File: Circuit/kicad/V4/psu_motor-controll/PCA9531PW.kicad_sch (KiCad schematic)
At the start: 15 parts, among them J1 Conn_01x12, U3 PCA9685PW

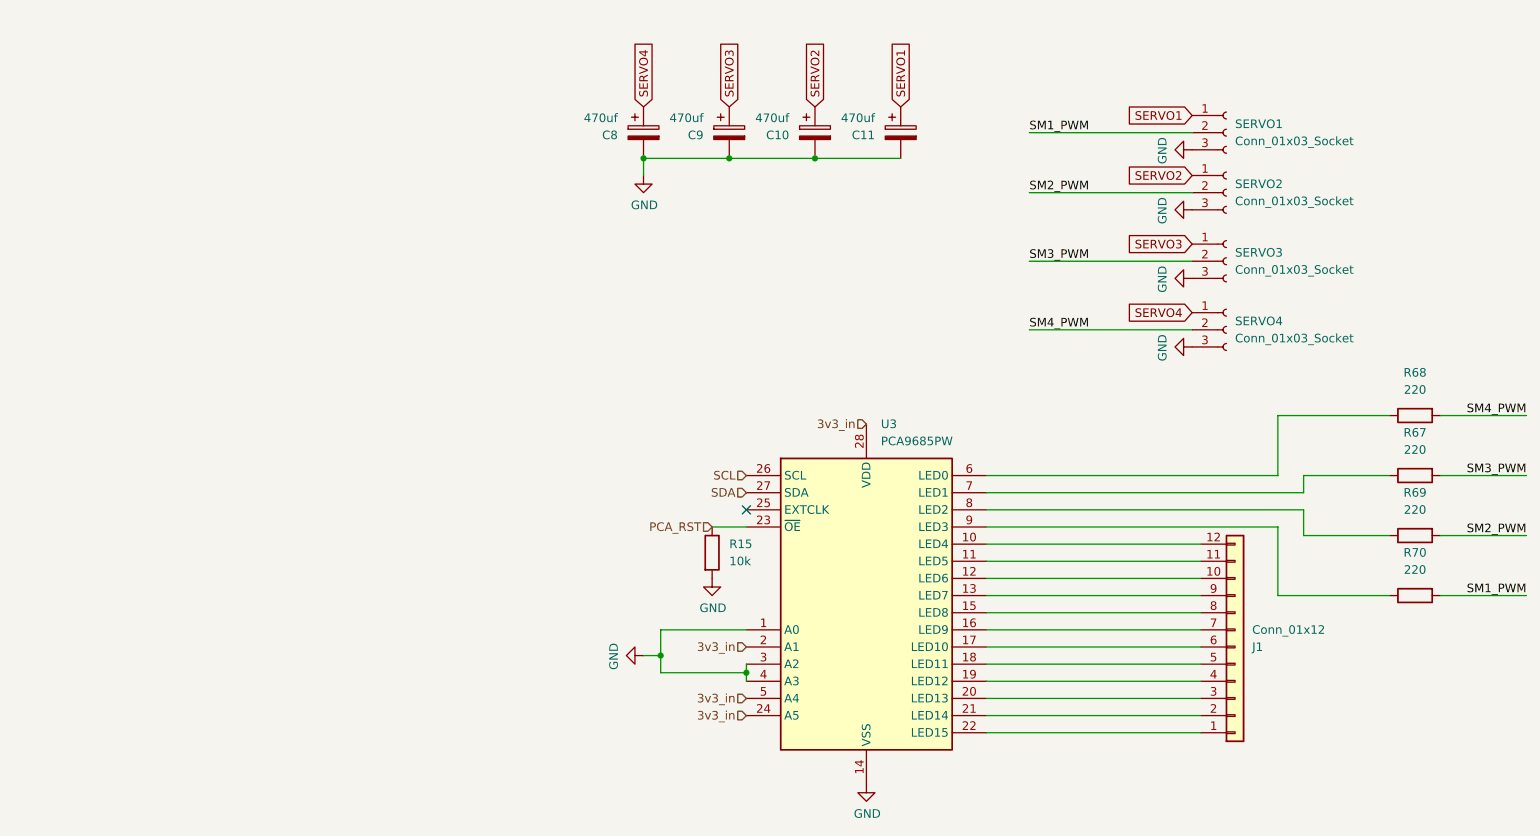
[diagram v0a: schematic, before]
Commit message: PSU FINISH BOARD NO DRC,ERC,DFM ERRORS
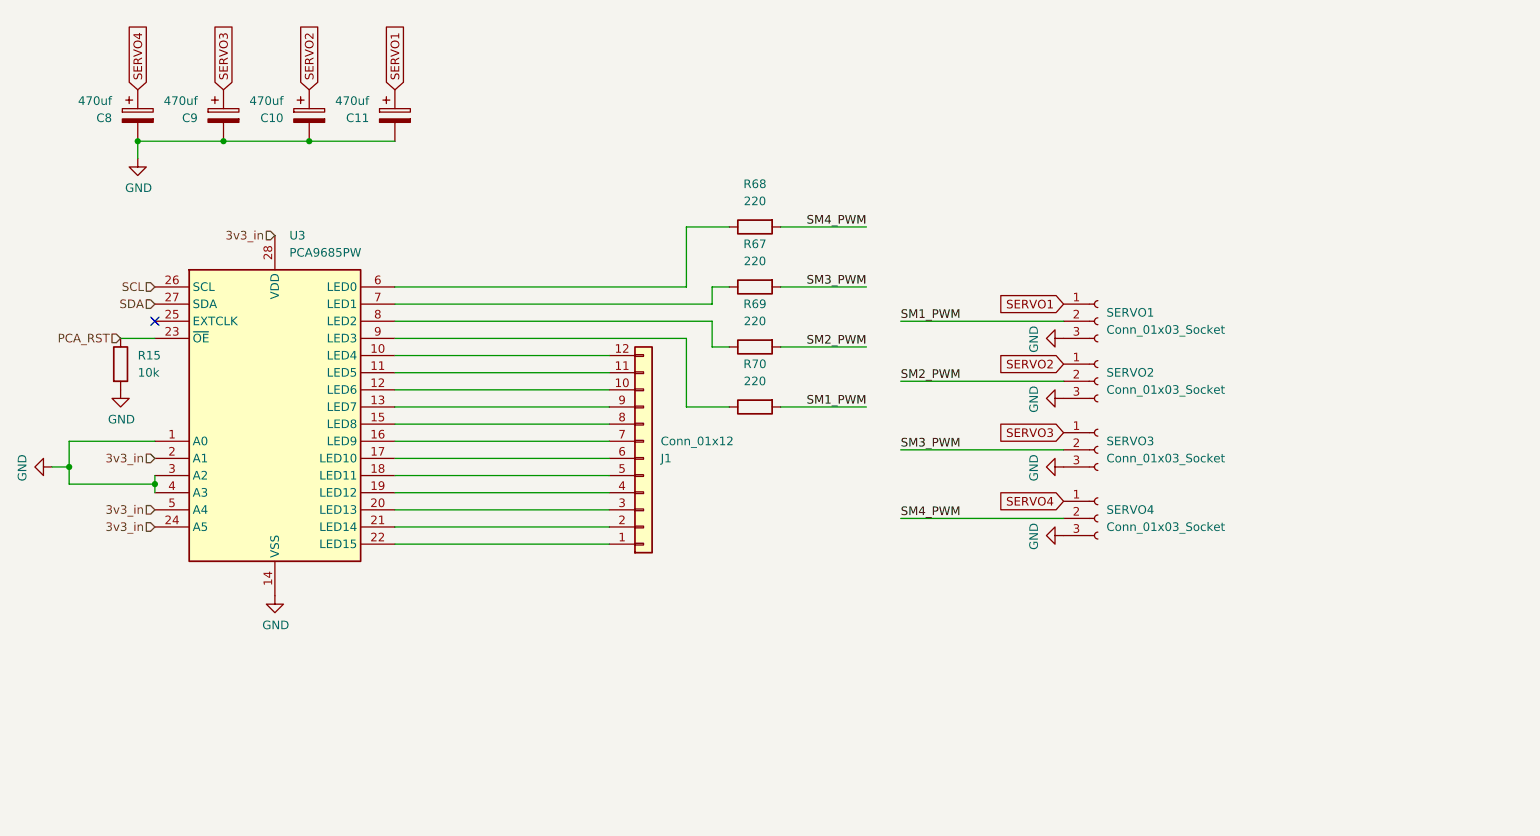
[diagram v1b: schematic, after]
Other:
- moved on the sheet: C10, C11, C8, C9, J1, R15, R67, R68, R69, R70, SERVO1, SERVO2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
